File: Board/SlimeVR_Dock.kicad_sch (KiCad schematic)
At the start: 25 parts, among them J1_Control Conn_01x03_Pin, J1_MainPW USB_C_Receptacle_USB2.0_16P, J1_Monitor Conn_01x03_Pin, J1_Prog Conn_01x03_Pin, M1 Fan, Q1 AO3401A, U1 ESP32-C3-WROOM-02, U17 74HC165, U18 74HC165, U19 74HC595, U2 CH224K, U3 XC6220B331MR

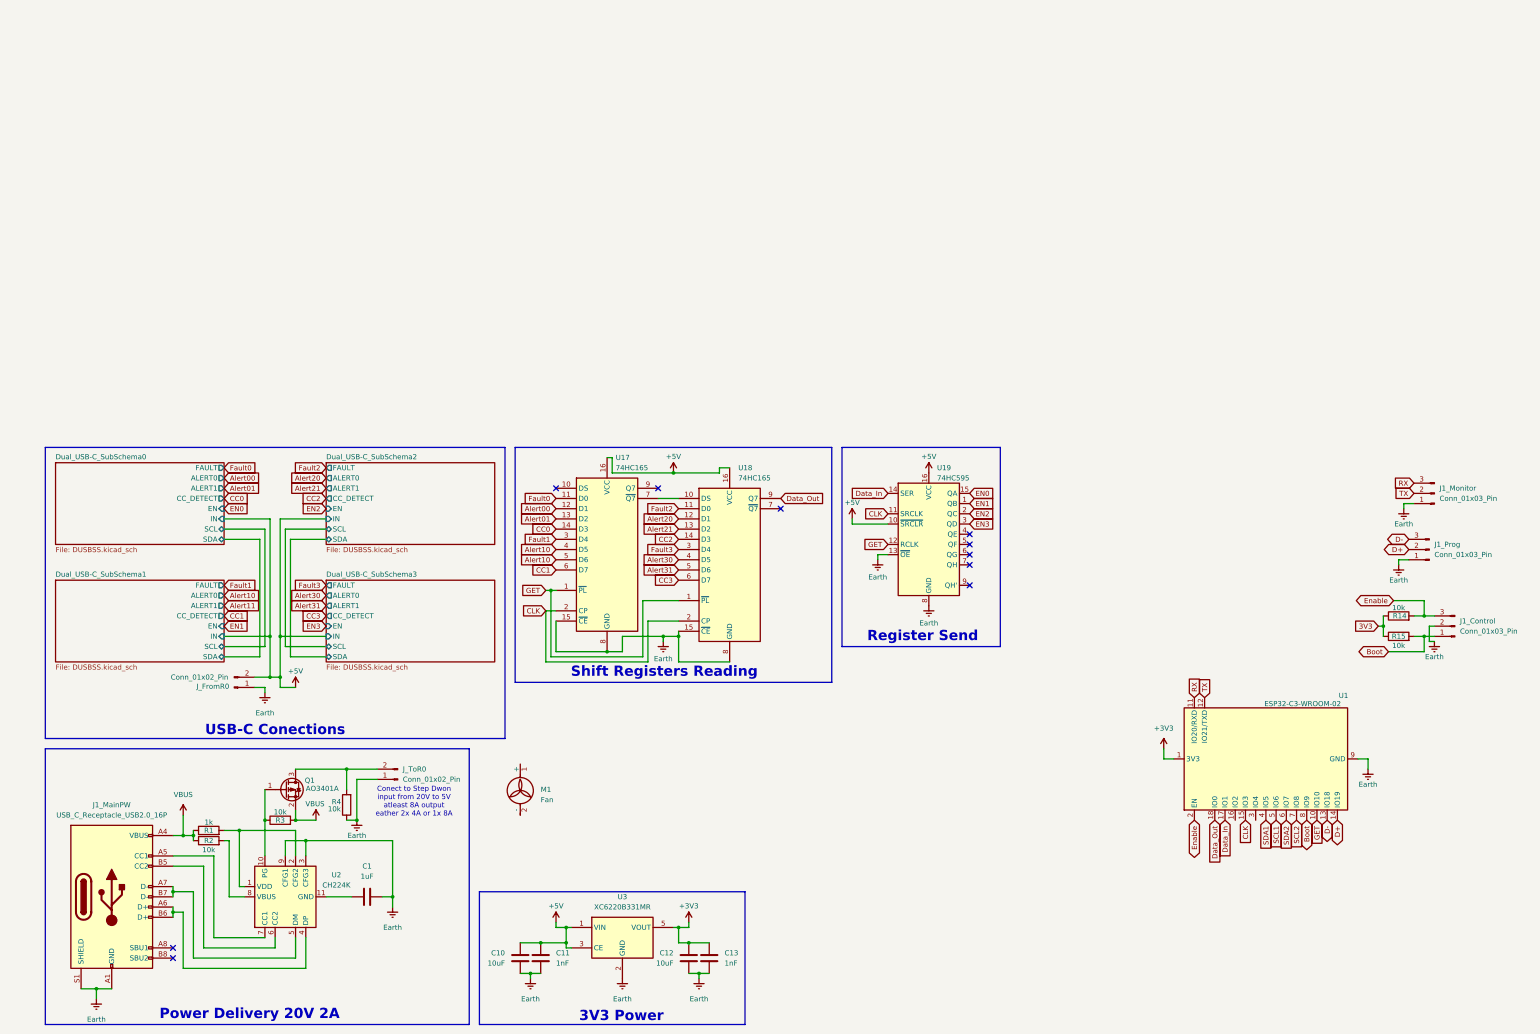
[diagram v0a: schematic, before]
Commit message: Finished Schematic
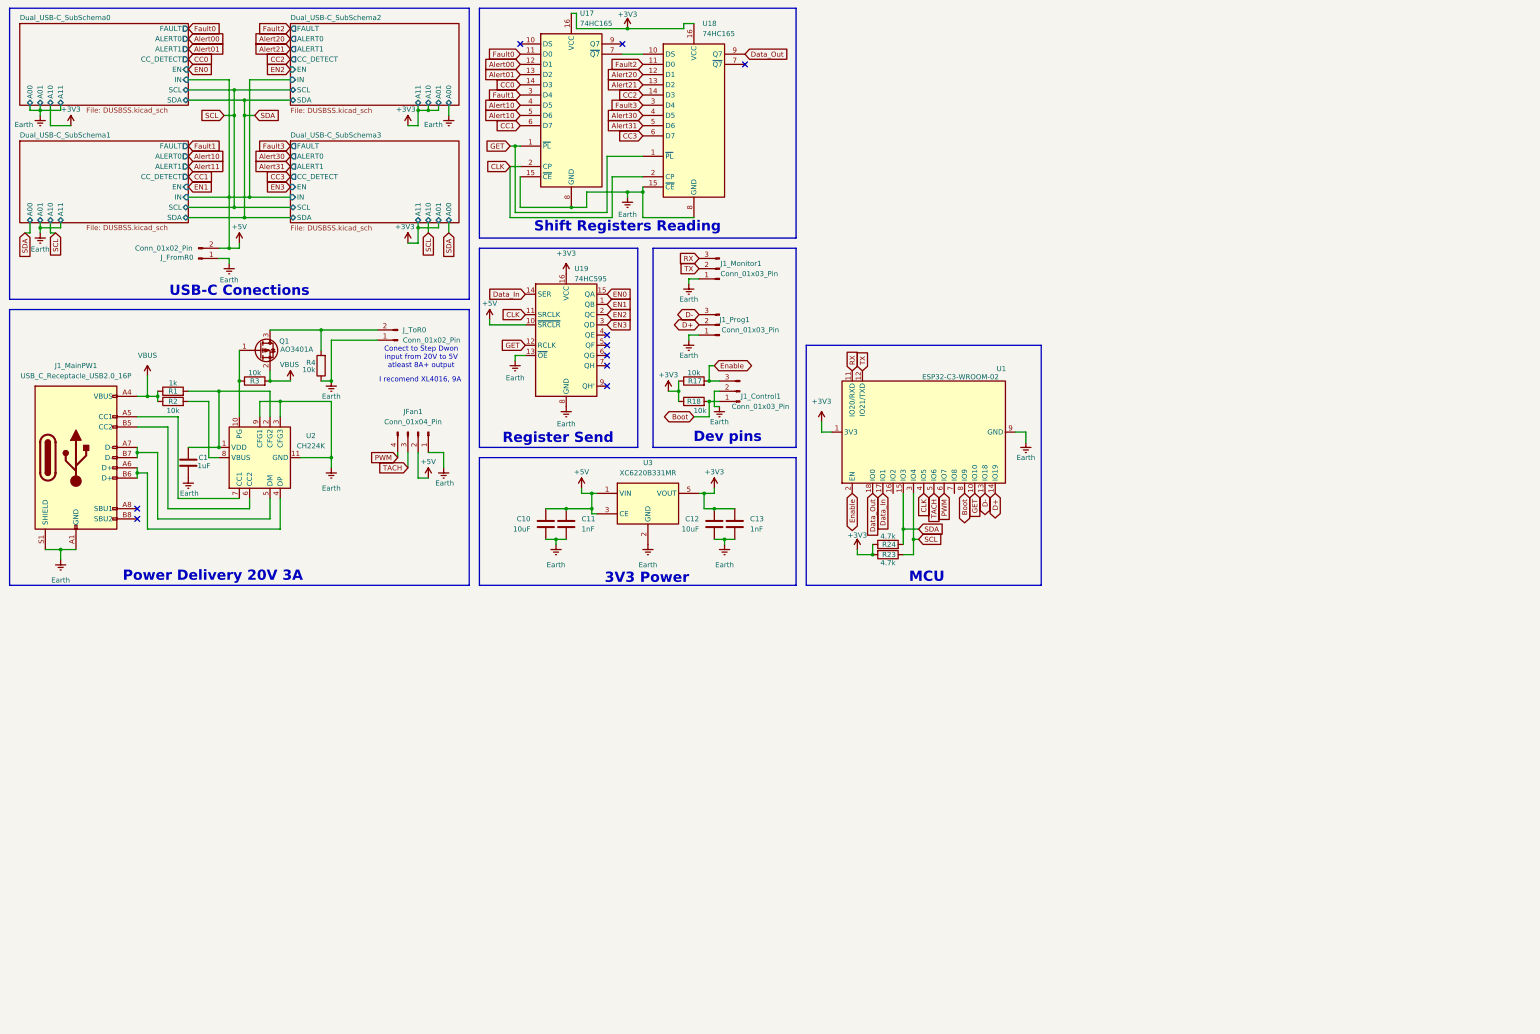
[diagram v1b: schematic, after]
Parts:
- removed M1: Fan, symbol Motor:Fan
- added JFan1: Conn_01x04_Pin, Connector:FanPinHeader_1x04_P2.54mm_Vertical, symbol Connector:Conn_01x04_Pin
- added R23, R24: 4.7k, Resistor_SMD:R_0603_1608Metric, symbol Device:R
- C1, C10, C11, C12, C13: footprint (none) -> Capacitor_SMD:C_0603_1608Metric
- J1_Control1: renamed from J1_Control; footprint (none) -> Connector_PinHeader_2.54mm:PinHeader_1x03_P2.54mm_Vertical
- J1_MainPW1: renamed from J1_MainPW; footprint (none) -> Connector_USB:USB_C_Receptacle_GCT_USB4105-xx-A_16P_TopMnt_Horizontal
- J1_Monitor1: renamed from J1_Monitor; footprint (none) -> Connector_PinHeader_2.54mm:PinHeader_1x03_P2.54mm_Vertical
- J1_Prog1: renamed from J1_Prog; footprint (none) -> Connector_PinHeader_2.54mm:PinHeader_1x03_P2.54mm_Vertical
- J_FromR0, J_ToR0: footprint (none) -> Connector_PinHeader_2.54mm:PinHeader_1x02_P2.54mm_Vertical
- R1, R2, R3, R4: footprint (none) -> Resistor_SMD:R_0603_1608Metric
- R17: renamed from R14; footprint (none) -> Resistor_SMD:R_0603_1608Metric
- R18: renamed from R15; footprint (none) -> Resistor_SMD:R_0603_1608Metric
- U17, U18, U19: footprint (none) -> Package_SO:SOIC-16_3.9x9.9mm_P1.27mm
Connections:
- net 3V3 is gone; now on net +3V3: R17.1, R18.1
- net SDA1 is gone; now on net CLK: U1.4 (IO5)
- net +3V3: now also U17.16 (VCC), U18.16 (VCC), U19.16 (VCC), R23.2, R24.1
- net +5V: now also JFan1.2 (Pin_2); no longer U17.16 (VCC), U18.16 (VCC), U19.16 (VCC)
- net CLK: no longer U1.15 (IO3)
- net Earth: now also C1.1, U2.11 (GND), JFan1.1 (Pin_1); no longer C1.2
- net SCL: now reaches U1.3 (IO4)
- net SCL: now also R23.1
- net at R1.2, U2.1 (VDD), U2.2 (CFG2): now also C1.2
- net SCL1 renamed TACH
- net TACH: now also JFan1.3 (Pin_3)
- net SCL2: no longer names the net of U1.7 (IO8)
- net SDA2 renamed PWM
- net PWM: now also JFan1.4 (Pin_4)
- new net SDA: R24.2, U1.15 (IO3)
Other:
- sheet Dual_USB-C_SubSchema0 ports: added A00, A01, A10, A11; removed none
- sheet Dual_USB-C_SubSchema1 ports: added A00, A01, A10, A11; removed none
- sheet Dual_USB-C_SubSchema2 ports: added A00, A01, A10, A11; removed none
- sheet Dual_USB-C_SubSchema3 ports: added A00, A01, A10, A11; removed none
- note added: "Conect to Step Dwon input from 20V to 5V atleast 8A+ output"
- note added: "Dev pins"
- note added: "I recomend XL4016, 9A"
- note added: "MCU"
- note added: "Power Delivery 20V 3A"
- note removed: "Conect to Step Dwon input from 20V to 5V atleast 8A output eather 2x 4A or 1x 8A"
- note removed: "Power Delivery 20V 2A"
- moved on the sheet: C1, C10, C11, C12, C13, J1_Control1, J1_MainPW1, J1_Monitor1, J1_Prog1, J_FromR0, J_ToR0, Q1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
